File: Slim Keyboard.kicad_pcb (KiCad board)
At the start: 2 copper layers, 25.5 x 46.5 mm, 63 parts, among them J1 USB_C_Receptacle_USB2.0_16P, J2 SWD, J3 SWC, J4 Conn_01x14_Pin, J5 S2B-PH-SM4-TB, J6 Conn_01x14_Pin, U1 NRF52840-QIAA-R, U2 BQ24075RGT, U3 XC6220B331MR, Y1 FC-12M 32.7680KA-AC0, Y2 XRCGB32M000F1S2KR0

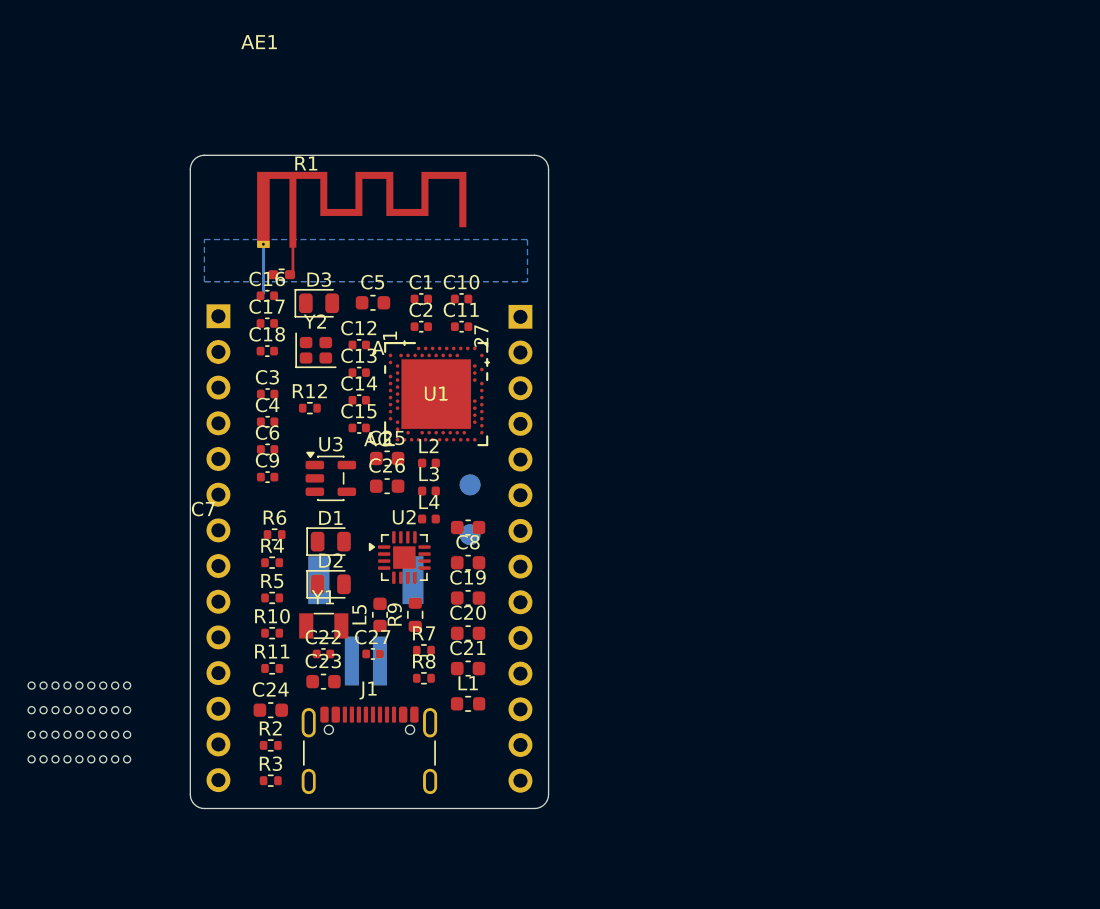
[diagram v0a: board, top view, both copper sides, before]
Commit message: Started PCB design
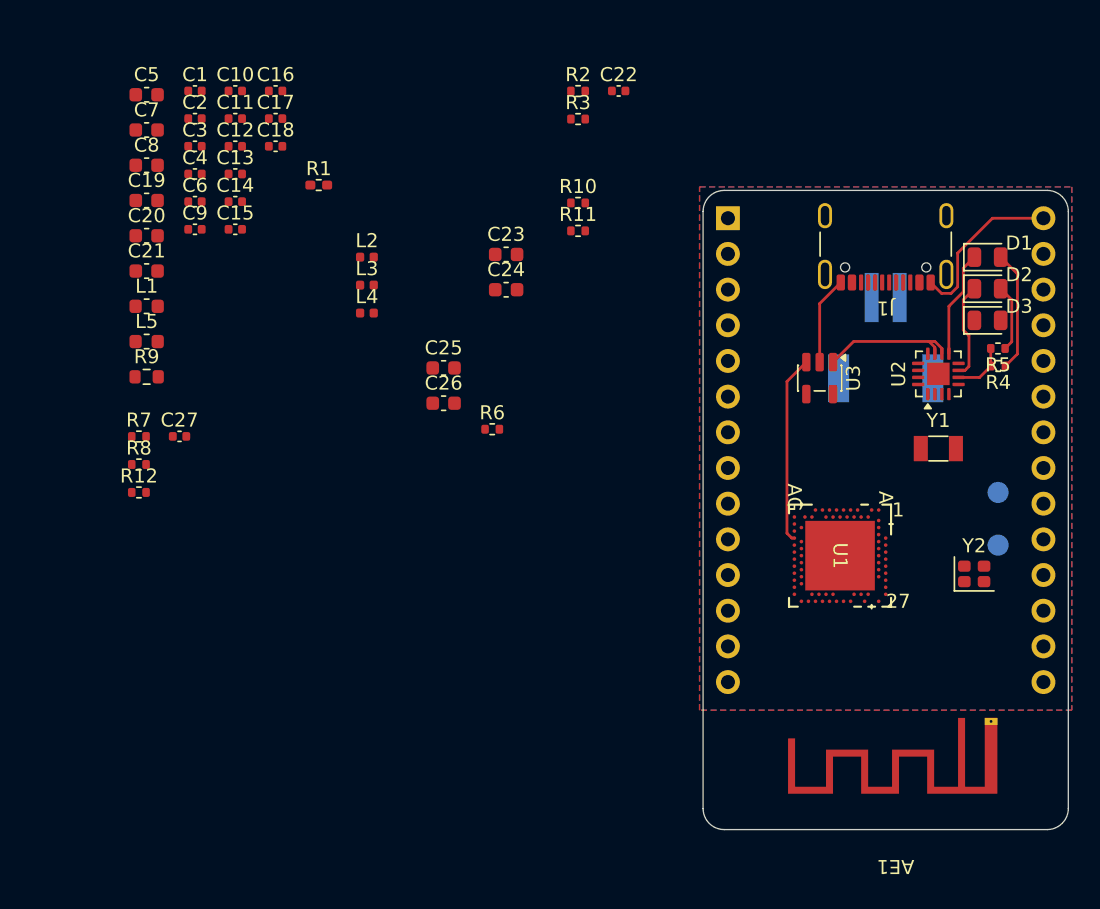
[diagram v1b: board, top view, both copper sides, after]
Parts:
- removed J4, J6: Conn_01x14_Pin, Connector_PinHeader_2.54mm:PinHeader_1x14_P2.54mm_Vertical
- removed rBT1, rBT2, rBT3, rBT4: Breakaway Tabs, Panelization:BreakLine_9h_D0.5mm_P0.85mm
- added J7: ~, KBSlim_NRF52840_module:NRF52840_module, F.Cu at (70.0, 40.2)
- C16: value 1pF -> 1.2pF
- D1: value Orange -> LTST-C170KFKT
- D2: value Green -> LTST-C170KGKT
- D3: value BLUE -> IN-S85AT5B
- R4, R5, R9: value R -> 1k
- Y1: value FC-12M 32.7680KA-AC0 -> ECS-.327-9-34B-TR
- moved AE1 68.8 mm to (91.0, 83.0), turned to 180 degrees
- moved R5 54.6 mm to (91.0, 51.2), turned to 180 degrees
- moved R4 53.5 mm to (91.0, 52.5), turned to 180 degrees
- moved J1 53.0 mm to (83.0, 42.9), turned to 180 degrees
- moved R3 51.9 mm to (61.1, 34.9)
- moved R2 51.5 mm to (61.1, 32.9)
- moved D2 51.3 mm to (90.2, 47.0)
- moved D1 50.9 mm to (90.2, 44.8)
- moved Y2 49.5 mm to (89.3, 67.3)
- moved D3 47.6 mm to (90.2, 49.2)
- moved Y1 45.5 mm to (86.8, 58.4)
- moved C22 45.3 mm to (64.0, 32.9)
- moved J5 45.1 mm to (83.0, 47.6), turned to 0 degrees
- moved U2 40.2 mm to (86.8, 53.1), turned to 90 degrees
- moved R11 38.0 mm to (61.1, 42.9)
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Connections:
- U1 pad AD10: unconnected-(U1-P0.15-PadAD10) -> BLED
- U1 pad AD8: unconnected-(U1-P0.13-PadAD8) -> POWER_PIN
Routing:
- net GND: track 3.75 -> 18.3 mm
- net VDDH: track 0.00 -> 13.9 mm
- net POWER_PIN: track 0.00 -> 13.4 mm
- net Net-(D1-A): track 0.00 -> 8.60 mm
- net Net-(D1-K): track 0.00 -> 7.63 mm
- net Net-(D2-K): track 0.00 -> 6.88 mm
- net Net-(D2-A): track 0.00 -> 4.77 mm
- net Net-(AE1-A): track 4.45 -> 0.00 mm
- added copper zone on F.Cu, net GND
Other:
- board size 25.5 x 46.5 mm -> 26 x 45.5 mm
